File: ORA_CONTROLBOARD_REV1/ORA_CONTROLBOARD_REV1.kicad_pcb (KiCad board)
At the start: 2 copper layers, 100 x 100 mm, 34 parts, among them J1 Screw_Terminal_01x02, J2 Screw_Terminal_01x02, J3 USB_B_Micro, Q1 FDN340P, U1 ATmega32U4-A, U2 MCP2515-xSO, U3 MCP2551-I-SN, U4 PMV48XP_215, U5 NCP1117-5.0_SOT223

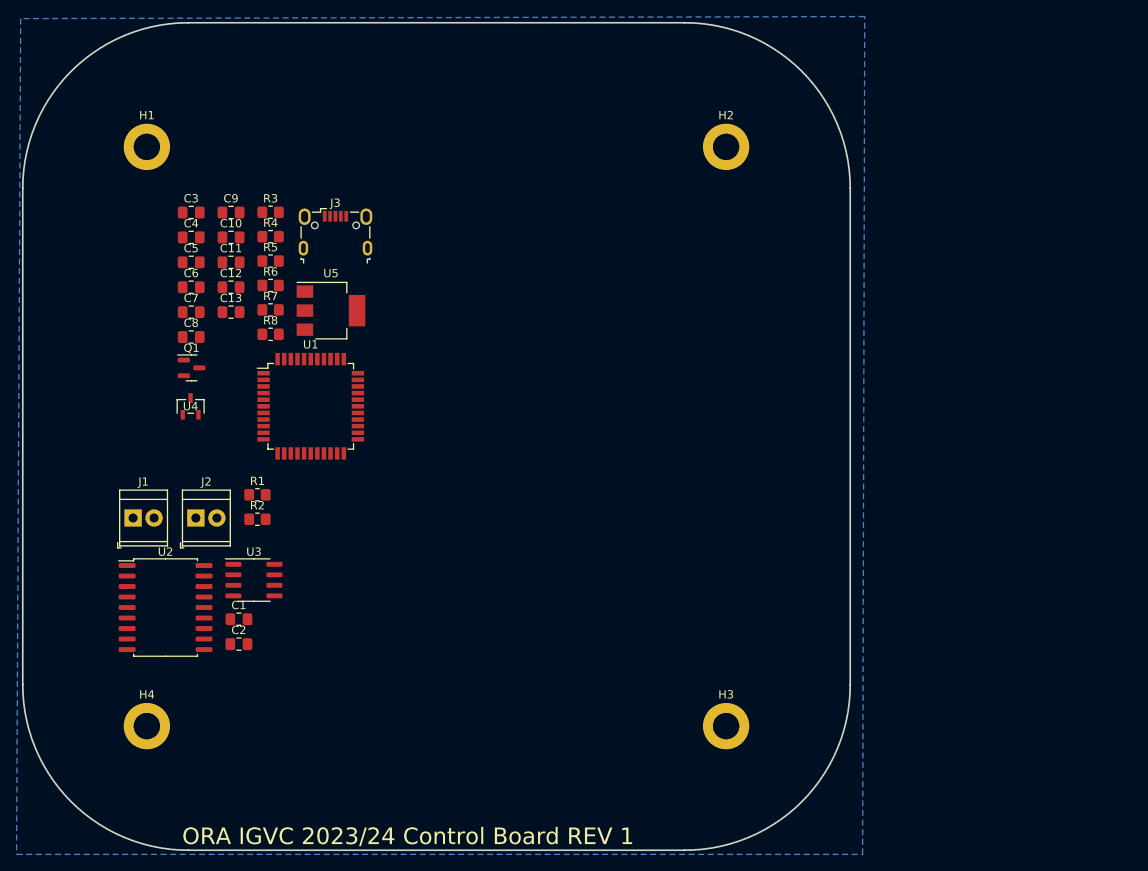
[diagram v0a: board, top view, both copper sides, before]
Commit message: I broke it
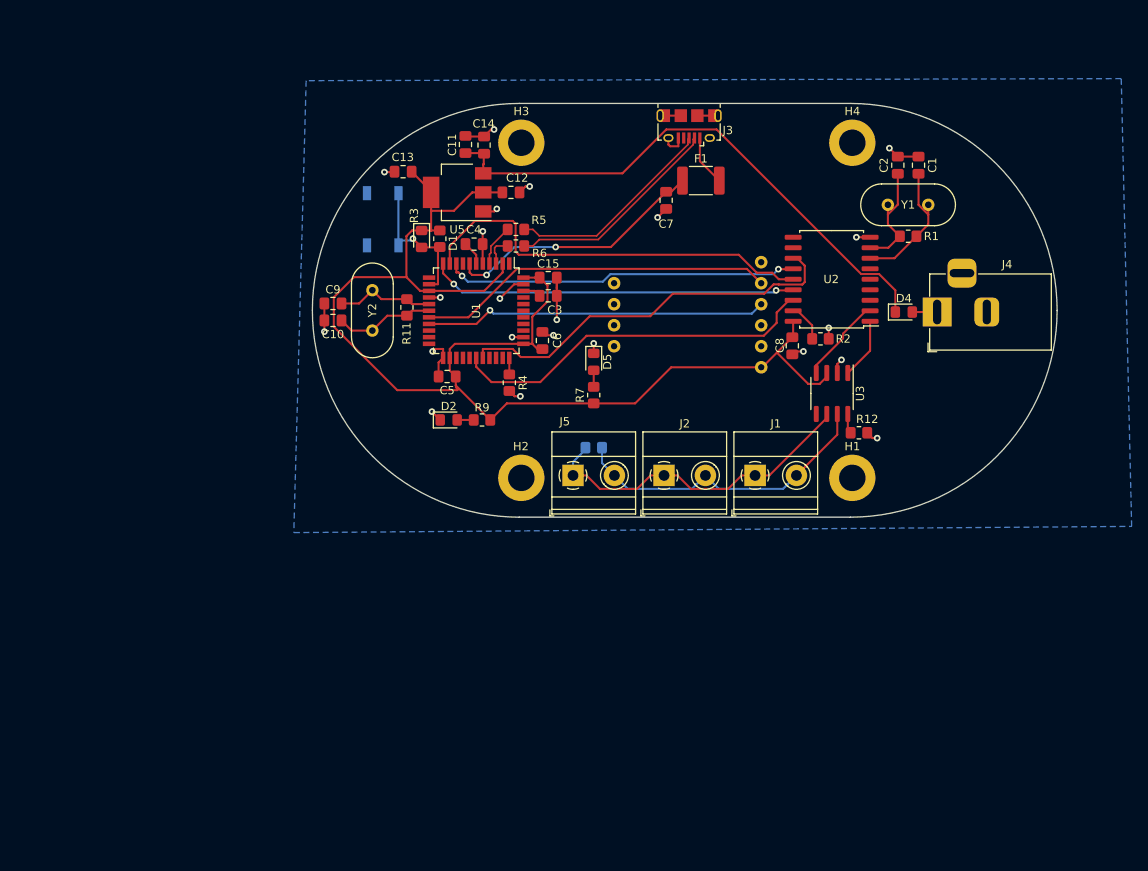
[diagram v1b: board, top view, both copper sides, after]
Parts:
- removed Q1: FDN340P, Package_TO_SOT_SMD:SOT-23
- removed R8: 10k, Resistor_SMD:R_0805_2012Metric_Pad1.20x1.40mm_HandSolder
- removed U4: PMV48XP_215, footprints:TO-236_SOT23_NEX
- added C14: 100nF, Capacitor_SMD:C_0805_2012Metric_Pad1.18x1.45mm_HandSolder, F.Cu at (120.8, 54.8)
- added C15: 1uF, Capacitor_SMD:C_0805_2012Metric_Pad1.18x1.45mm_HandSolder, F.Cu at (128.5, 70.8)
- added D1: rst, Diode_SMD:D_0805_2012Metric_Pad1.15x1.40mm_HandSolder, F.Cu at (113.2, 66.1)
- added D2: LED_Small, LED_SMD:LED_0805_2012Metric_Pad1.15x1.40mm_HandSolder, F.Cu at (116.5, 88.0)
- added D4: PWRIN, Diode_SMD:D_0805_2012Metric_Pad1.15x1.40mm_HandSolder, F.Cu at (171.5, 75.0)
- added D5: IMU_LED, LED_SMD:LED_0805_2012Metric_Pad1.15x1.40mm_HandSolder, F.Cu at (134.0, 81.0)
- added F1: MF-MSMF050-2, Fuse:Fuse_1812_4532Metric_Pad1.30x3.40mm_HandSolder, F.Cu at (146.9, 59.1)
- added J4: PW IN, Connector_BarrelJack:BarrelJack_Horizontal, F.Cu at (175.5, 75.0)
- added J5: CAN, TerminalBlock_Phoenix:TerminalBlock_Phoenix_MKDS-1,5-2_1x02_P5.00mm_Horizontal, F.Cu at (131.5, 94.7)
- added R11: 1M, Resistor_SMD:R_0805_2012Metric_Pad1.20x1.40mm_HandSolder, F.Cu at (111.4, 74.4)
- added R12: 10k, Resistor_SMD:R_0805_2012Metric_Pad1.20x1.40mm_HandSolder, F.Cu at (166.1, 89.5)
- added R13: 120, Resistor_SMD:R_0805_2012Metric_Pad1.20x1.40mm_HandSolder, B.Cu at (134.0, 91.3)
- added R9: 470, Resistor_SMD:R_0805_2012Metric_Pad1.20x1.40mm_HandSolder, F.Cu at (120.5, 88.0)
- added SW1: Reset, Button_Switch_SMD:SW_SPST_TL3342, B.Cu at (108.5, 63.8)
- added U6: IMU_MOUNT, Custom_Parts:IMU_MOUNT, F.Cu at (135.2, 88.0)
- added Y1: 8Mhz, Crystal:Crystal_HC49-4H_Vertical, F.Cu at (169.6, 62.0)
- added Y2: 16MHz, Crystal:Crystal_HC49-4H_Vertical, F.Cu at (107.2, 77.2)
- C11: value 100uF -> 10nF
- C7: value 22uF -> 100nF
- J1, J2: value Screw_Terminal_01x02 -> CAN; footprint TerminalBlock_TE-Connectivity:TerminalBlock_TE_282834-2_1x02_P2.54mm_Horizontal -> TerminalBlock_Phoenix:TerminalBlock_Phoenix_MKDS-1,5-2_1x02_P5.00mm_Horizontal
- J3: footprint Connector_USB:USB_Micro-B_Wuerth_629105150521 -> Connector_USB:USB_Micro-B_Amphenol_10118194_Horizontal
- R1: value 10k -> 1M
- R7: value 10k -> 470
- moved H4 110.6 mm to (165.2, 54.5)
- moved C1 98.8 mm to (173.2, 57.2), turned to -90 degrees
- moved C2 98.4 mm to (170.8, 57.2), turned to 90 degrees
- moved H1 94.2 mm to (165.2, 95.0)
- moved U2 89.7 mm to (162.8, 71.0), turned to 180 degrees
- moved R1 84.6 mm to (172.0, 65.8), turned to 180 degrees
- moved J1 75.3 mm to (153.5, 94.7)
- moved H3 74.7 mm to (125.2, 54.5)
- moved U3 73.4 mm to (162.8, 84.8), turned to -90 degrees
- moved C8 72.6 mm to (158.0, 79.0), turned to -90 degrees
- moved R2 71.4 mm to (161.4, 78.2), turned to 180 degrees
- moved C7 59.0 mm to (142.8, 61.5), turned to -90 degrees
- moved J2 56.8 mm to (142.5, 94.7)
- moved H2 47.0 mm to (125.2, 95.0)
- moved J3 44.6 mm to (145.5, 52.5), turned to 180 degrees
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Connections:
- net Net-(J3-D+) renamed (USB) D+
- net Net-(J3-D-) renamed (USB) D-
- net Net-(U4-S) renamed PWRIN
- C7 pad 1: Net-(J3-VBUS) -> VBUS
- C8 pad 1: Vusb -> +5V
- J1 pad 1: CAN_H -> CAN_L
- J1 pad 2: CAN_L -> CAN_H
- J2 pad 1: CAN_H -> CAN_L
- J2 pad 2: CAN_L -> CAN_H
- R1 pad 1: Net-(U3-Rs) -> Net-(U2-OSC2)
- R1 pad 2: GND -> Net-(U2-OSC1)
- R7 pad 1: Vusb -> +5V
- R7 pad 2: GND -> Net-(D5-A)
- U1 pad 10: unconnected-(U1-PB2-Pad10) -> CAN_SI
- U1 pad 11: unconnected-(U1-PB3-Pad11) -> CAN_SO
- U1 pad 18: unconnected-(U1-PD0-Pad18) -> IMU_SCL
- U1 pad 19: unconnected-(U1-PD1-Pad19) -> IMU_SDA
- U1 pad 28: unconnected-(U1-PB4-Pad28) -> CAN_CS
- U1 pad 29: unconnected-(U1-PB5-Pad29) -> CAN_INT
- U1 pad 3: unconnected-(U1-D--Pad3) -> D-
- U1 pad 4: unconnected-(U1-D+-Pad4) -> D+
- U1 pad 7: unconnected-(U1-VBUS-Pad7) -> VBUS
- U1 pad 9: unconnected-(U1-PB1-Pad9) -> CAN_SCK
- U3 pad 1: Net-(U2-RXCAN) -> Net-(U2-TXCAN)
- U3 pad 4: Net-(U2-TXCAN) -> Net-(U2-RXCAN)
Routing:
- net +5V: track 0.00 -> 158.6 mm
- net PWRIN: track 0.00 -> 67.4 mm
- net GND: track 0.00 -> 60.6 mm, vias 0 -> 22
- net CAN_SI: track 0.00 -> 49.8 mm
- net CAN_INT: track 0.00 -> 47.9 mm
- net CAN_CS: track 0.00 -> 45.0 mm
- net CAN_SO: track 0.00 -> 44.6 mm, vias 0 -> 2
- net IMU_SCL: track 0.00 -> 43.3 mm
- net CAN_SCK: track 0.00 -> 42.9 mm, vias 0 -> 2
- net IMU_SDA: track 0.00 -> 41.5 mm, vias 0 -> 1
- net CAN_L: track 0.00 -> 40.7 mm
- net CAN_H: track 0.00 -> 38.1 mm
- net VBUS: track 0.00 -> 31.6 mm, vias 0 -> 2
- net (USB) D-: track 0.00 -> 26.4 mm
- net (USB) D+: track 0.00 -> 25.5 mm
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- added copper zone on B.Cu, net GND
- removed copper zone on B.Cu, net XTAL1
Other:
- board size 100 x 100 mm -> 90 x 50 mm
- board text added: "11/24/2023"
- board text added: "Add if terminating"
- board text added: "H"
- board text added: "L"
- board text added: "https://github.com/AndrewMcGhee"
